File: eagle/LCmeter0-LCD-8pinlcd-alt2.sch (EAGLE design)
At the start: 34 parts, among them IC1 PIC16F876A-X/SP, J1 HD44780-4BIT-8PIN, J2 PIC-UART, J3 PIC-ICSP, K2 DS2Y, Q1 20MHz, T1 BC547CBE-A, X1 FREQ, X2 L/C

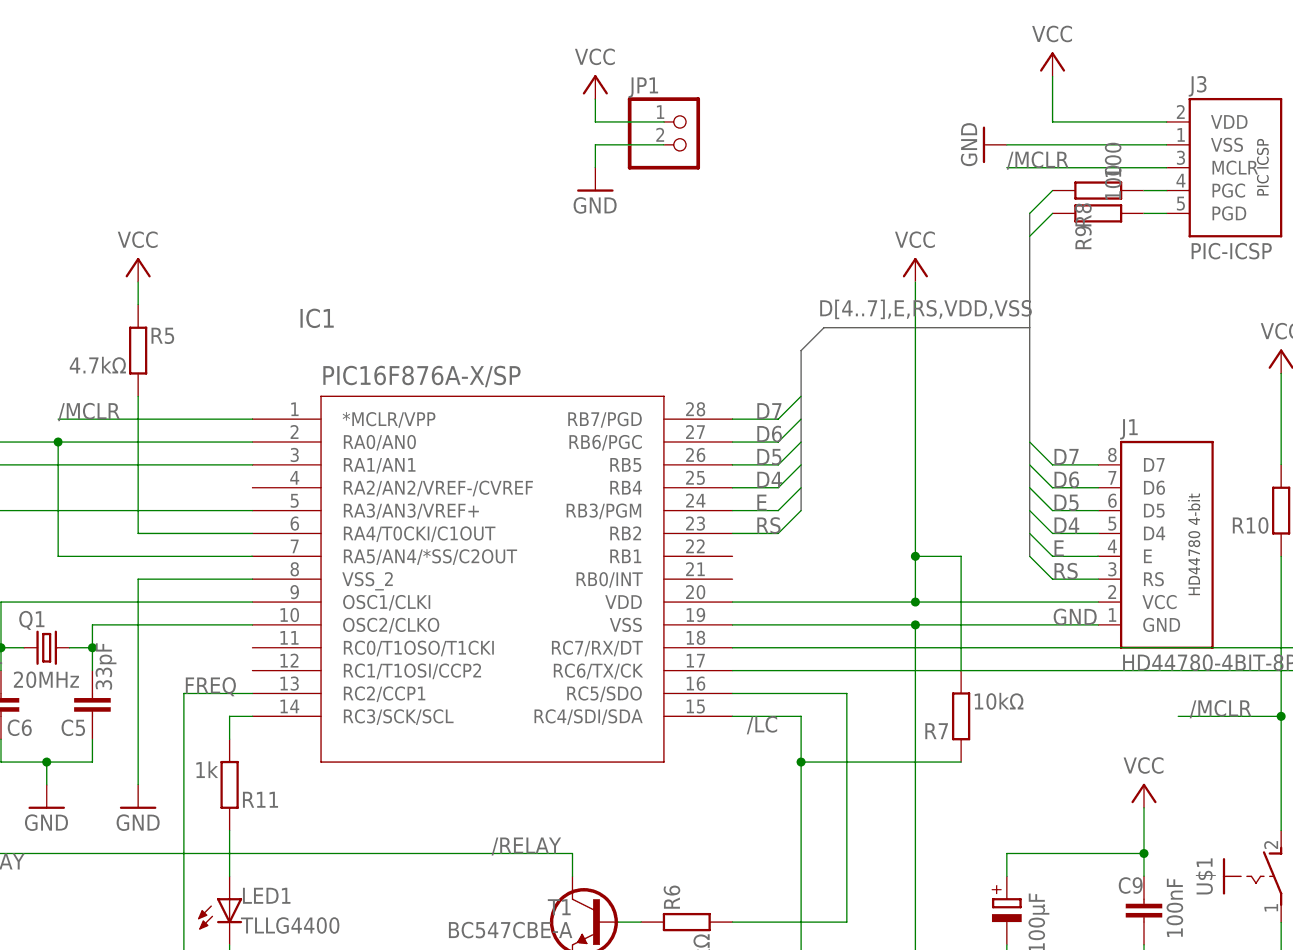
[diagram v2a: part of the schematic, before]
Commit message: ...
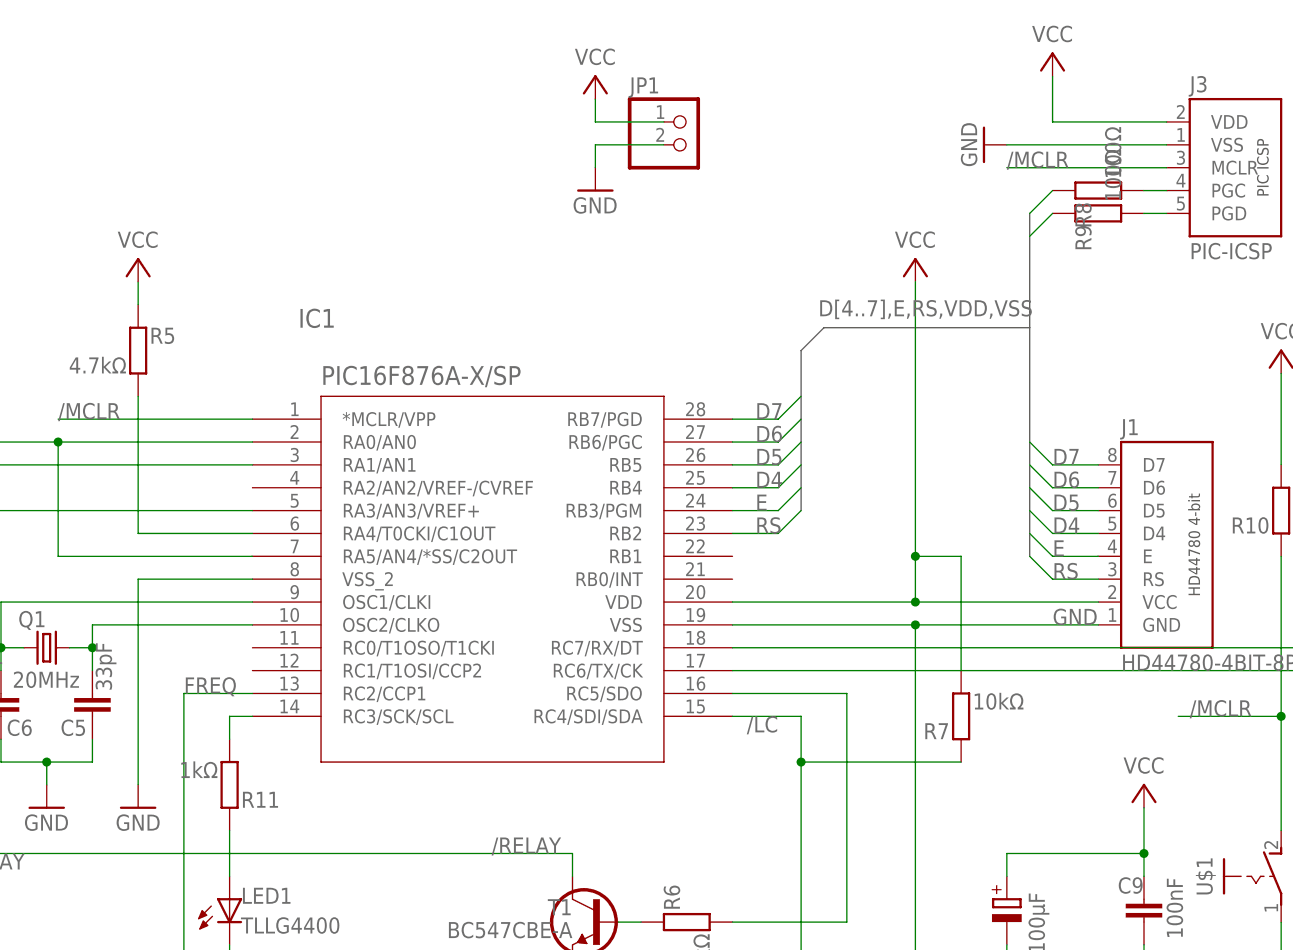
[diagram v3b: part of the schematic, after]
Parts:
- R11: value 1k -> 1kΩ
- R8, R9: value 100 -> 100Ω
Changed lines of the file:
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@@
 <part name="P+1" library="supply1" deviceset="VCC" device=""/>
 <part name="GND9" library="supply1" deviceset="GND" device=""/>
-<part name="R8" library="r" deviceset="R" device="0202/5" value="100"/>
-<part name="R9" library="r" deviceset="R" device="0202/5" value="100"/>
+<part name="R8" library="r" deviceset="R" device="0202/5" value="100Ω"/>
+<part name="R9" library="r" deviceset="R" device="0202/5" value="100Ω"/>
 <part name="J1" library="pinconn" deviceset="HD44780-4BIT" device="-8PIN"/>
-<part name="R11" library="r" deviceset="R" device="0202/5" value="1k"/>
+<part name="R11" library="r" deviceset="R" device="0202/5" value="1kΩ"/>
 <part name="LED1" library="led" deviceset="TLLG4400" device=""/>
 <part name="GND10" library="supply1" deviceset="GND" device=""/>
